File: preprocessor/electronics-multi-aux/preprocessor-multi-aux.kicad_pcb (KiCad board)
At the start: 2 copper layers, 17 x 24 mm, 19 parts, among them P1 ST-IN, P2 ST-OUT, P3 TH-IN, P4 TH-OUT, P5 AUX-IN, P6 LIGHT CONTROLLER, P7 AUX2-IN, P8 AUX3-IN, U1 MCP1703T-3302E/CB, U2 LPC811M001JDH16_TSSOP16

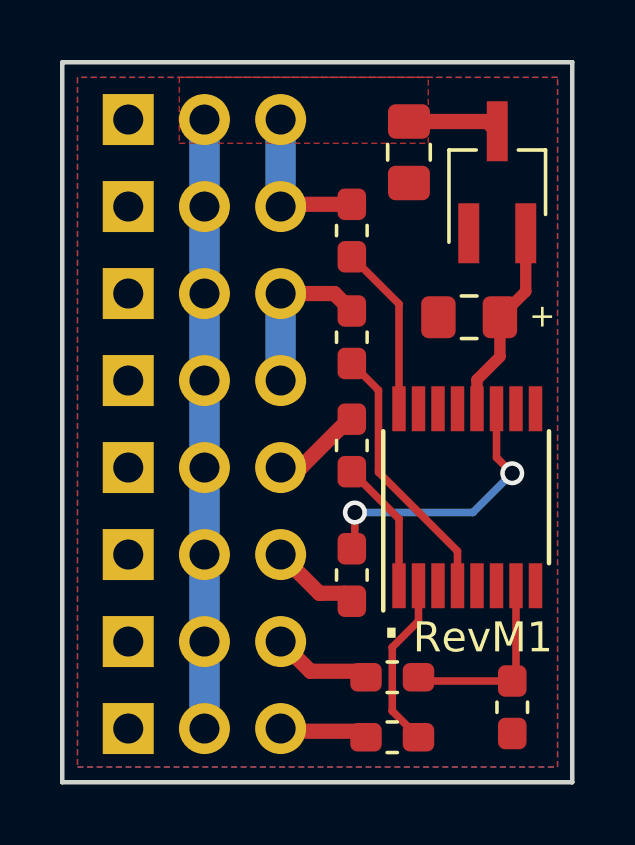
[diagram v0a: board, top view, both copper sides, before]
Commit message: Add to design doc and tweak PCB
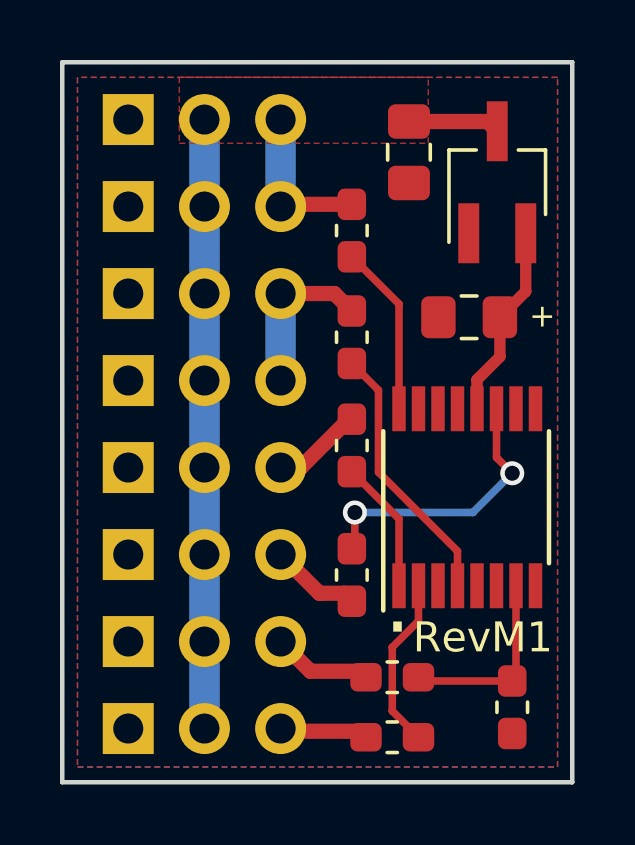
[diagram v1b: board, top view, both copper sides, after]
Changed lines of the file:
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@@
     (34 B.Paste user hide)
     (35 F.Paste user)
-    (36 B.SilkS user)
+    (36 B.SilkS user hide)
     (37 F.SilkS user)
     (38 B.Mask user hide)
@@
   )
   (setup
-    (last_trace_width 1.016)
+    (last_trace_width 0.254)
     (user_trace_width 0.381)
     (user_trace_width 0.508)
@@
     )
   )
-  (gr_text . (at 125.2728 60.2996) (layer F.SilkS)
+  (gr_text . (at 125.476 60.0964) (layer F.SilkS)
     (effects (font (size 2 2) (thickness 0.4)))
   )

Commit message: Update design doc
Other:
- board text added: "Note: pin headers spaced at 2.9mm to clear plug being wider on the top"
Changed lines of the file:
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@@
   (general
     (thickness 1.6)
-    (drawings 23)
+    (drawings 24)
     (tracks 56)
     (zones 0)
@@
     )
   )
+  (gr_text "Note: pin headers spaced at 2.9mm \nto clear plug being wider on the top" (at 98.552 53.2892) (layer Cmts.User)
+    (effects (font (size 1 1) (thickness 0.25)))
+  )
   (gr_text . (at 125.476 60.0964) (layer F.SilkS)

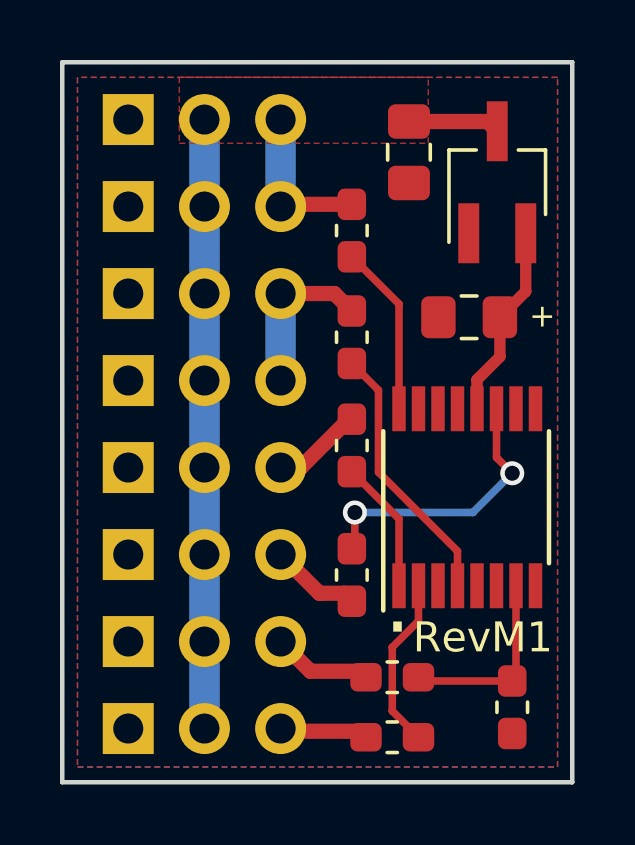
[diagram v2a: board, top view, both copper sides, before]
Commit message: Tweak tracks
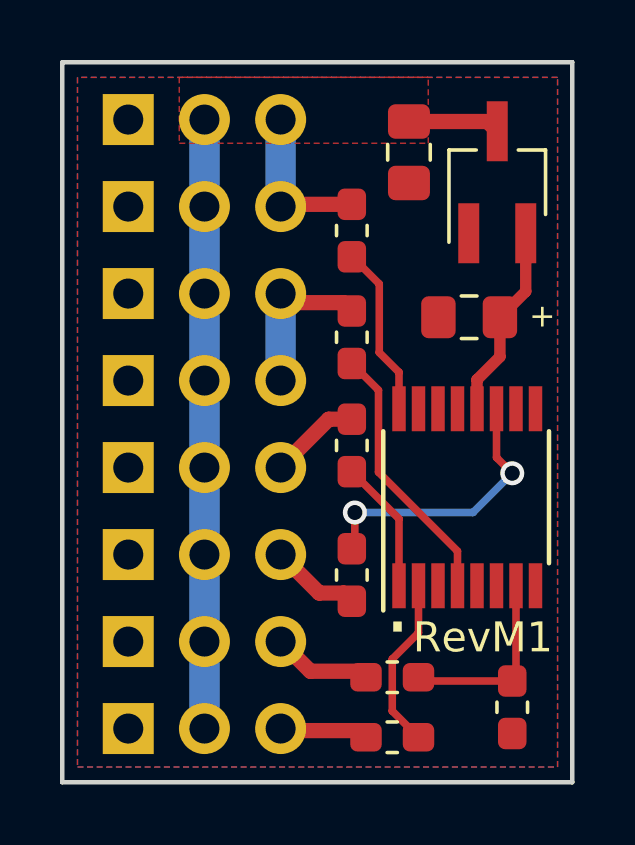
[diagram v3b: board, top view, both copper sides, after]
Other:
- rule pad_to_mask_clearance: 0.0508 -> 0.0254
- rule solder_mask_min_width: 0.0508 -> 0.0254
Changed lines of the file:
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@@
     (thickness 1.6)
     (drawings 24)
-    (tracks 56)
+    (tracks 60)
     (zones 0)
     (modules 19)
@@
     (34 B.Paste user hide)
     (35 F.Paste user)
-    (36 B.SilkS user hide)
+    (36 B.SilkS user)
     (37 F.SilkS user)
     (38 B.Mask user hide)
@@
     (pad_size 1.524 1.524)
     (pad_drill 0.762)
-    (pad_to_mask_clearance 0.0508)
-    (solder_mask_min_width 0.0508)
+    (pad_to_mask_clearance 0.0254)
+    (solder_mask_min_width 0.0254)
     (pad_to_paste_clearance_ratio -0.05)
     (aux_axis_origin 114.3 66.04)
@@
   (segment (start 128.125 52.6214) (end 128.8886 51.8578) (width 0.381) (layer F.Cu) (net 3))
   (segment (start 121.58 43.95) (end 121.58 46.85) (width 1.016) (layer B.Cu) (net 4))
+  (segment (start 123.952 46.7754) (end 121.6546 46.7754) (width 0.508) (layer F.Cu) (net 4))
   (segment (start 121.6546 46.7754) (end 121.58 46.85) (width 0.508) (layer F.Cu) (net 4))
-  (segment (start 123.952 46.7754) (end 121.6546 46.7754) (width 0.508) (layer F.Cu) (net 4))
   (segment (start 121.58 49.75) (end 121.58 52.65) (width 1.016) (layer B.Cu) (net 5))
-  (segment (start 123.3706 49.75) (end 123.952 50.3314) (width 0.508) (layer F.Cu) (net 5))
-  (segment (start 121.58 49.75) (end 123.3706 49.75) (width 0.508) (layer F.Cu) (net 5))
-  (segment (start 122.25 55.55) (end 121.58 55.55) (width 0.508) (layer F.Cu) (net 6))
-  (segment (start 123.952 53.9382) (end 123.8618 53.9382) (width 0.508) (layer F.Cu) (net 6))
-  (segment (start 123.8618 53.9382) (end 122.25 55.55) (width 0.508) (layer F.Cu) (net 6))
-  (segment (start 121.67 64.34) (end 121.58 64.25) (width 0.508) (layer F.Cu) (net 7))
-  (segment (start 124.425 64.54) (end 124.225 64.34) (width 0.508) (layer F.Cu) (net 7))
-  (segment (start 124.225 64.34) (end 121.67 64.34) (width 0.508) (layer F.Cu) (net 7))
-  (segment (start 125.525 50.0984) (end 125.525 53.59) (width 0.254) (layer F.Cu) (net 8))
-  (segment (start 123.952 48.5254) (end 125.525 50.0984) (width 0.254) (layer F.Cu) (net 8))
+  (segment (start 121.58 49.75) (end 121.88324 50.05324) (width 0.508) (layer F.Cu) (net 5))
+  (segment (start 123.67384 50.05324) (end 123.952 50.3314) (width 0.508) (layer F.Cu) (net 5))
+  (segment (start 121.88324 50.05324) (end 123.67384 50.05324) (width 0.508) (layer F.Cu) (net 5))
+  (segment (start 121.58 55.53928) (end 121.58 55.55) (width 0.508) (layer F.Cu) (net 6))
+  (segment (start 123.952 53.9382) (end 123.18108 53.9382) (width 0.508) (layer F.Cu) (net 6))
+  (segment (start 123.18108 53.9382) (end 121.58 55.53928) (width 0.508) (layer F.Cu) (net 6))
+  (segment (start 121.64788 64.31788) (end 121.58 64.25) (width 0.508) (layer F.Cu) (net 7))
+  (segment (start 124.425 64.54) (end 124.20288 64.31788) (width 0.508) (layer F.Cu) (net 7))
+  (segment (start 124.20288 64.31788) (end 121.64788 64.31788) (width 0.508) (layer F.Cu) (net 7))
+  (segment (start 125.525 52.373) (end 125.525 53.59) (width 0.254) (layer F.Cu) (net 8))
+  (segment (start 124.8664 49.4284) (end 124.8664 51.7144) (width 0.254) (layer F.Cu) (net 8))
+  (segment (start 124.8664 51.7144) (end 125.525 52.373) (width 0.254) (layer F.Cu) (net 8))
+  (segment (start 123.952 48.5254) (end 123.9634 48.5254) (width 0.254) (layer F.Cu) (net 8))
+  (segment (start 123.9634 48.5254) (end 124.8664 49.4284) (width 0.254) (layer F.Cu) (net 8))
   (segment (start 127.475 59.49) (end 127.475 58.3362) (width 0.254) (layer F.Cu) (net 9))
   (segment (start 127.475 58.3362) (end 124.841 55.7022) (width 0.254) (layer F.Cu) (net 9))
@@
   (segment (start 125.525 57.2612) (end 125.525 59.49) (width 0.254) (layer F.Cu) (net 10))
   (segment (start 123.952 55.6882) (end 125.525 57.2612) (width 0.254) (layer F.Cu) (net 10))
-  (segment (start 126.175 59.49) (end 126.175 60.665) (width 0.254) (layer F.Cu) (net 11))
-  (segment (start 126.175 60.665) (end 125.3 61.54) (width 0.254) (layer F.Cu) (net 11))
   (segment (start 125.3 63.665) (end 126.175 64.54) (width 0.254) (layer F.Cu) (net 11))
-  (segment (start 125.3 61.54) (end 125.3 63.665) (width 0.254) (layer F.Cu) (net 11))
-  (segment (start 122.8708 59.7408) (end 121.58 58.45) (width 0.508) (layer F.Cu) (net 12))
-  (segment (start 123.952 60.0062) (end 123.6866 59.7408) (width 0.508) (layer F.Cu) (net 12))
-  (segment (start 123.6866 59.7408) (end 122.8708 59.7408) (width 0.508) (layer F.Cu) (net 12))
+  (segment (start 125.3 61.93356) (end 125.3 63.665) (width 0.254) (layer F.Cu) (net 11))
+  (segment (start 126.175 59.49) (end 126.175 61.05856) (width 0.254) (layer F.Cu) (net 11))
+  (segment (start 126.175 61.05856) (end 125.3 61.93356) (width 0.254) (layer F.Cu) (net 11))
+  (segment (start 122.86318 59.73318) (end 121.58 58.45) (width 0.508) (layer F.Cu) (net 12))
+  (segment (start 123.952 60.0062) (end 123.67898 59.73318) (width 0.508) (layer F.Cu) (net 12))
+  (segment (start 123.67898 59.73318) (end 122.86318 59.73318) (width 0.508) (layer F.Cu) (net 12))
   (via (at 129.3 55.74) (size 0.8) (drill 0.5) (layers F.Cu B.Cu) (net 13))
   (segment (start 128.775 55.215) (end 128.775 53.59) (width 0.254) (layer F.Cu) (net 13))

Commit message: Add PCB thickness annotation
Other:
- board text added: "Thickness: 1mm"
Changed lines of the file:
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@@
   (general
     (thickness 1.6)
-    (drawings 24)
+    (drawings 25)
     (tracks 60)
     (zones 0)
@@
     )
   )
+  (gr_text "Thickness: 1mm" (at 99.06 39.37) (layer Cmts.User)
+    (effects (font (size 1.5 1.5) (thickness 0.3)))
+  )
   (gr_text "Note: pin headers spaced at 2.9mm \nto clear plug being wider on the top" (at 98.552 53.2892) (layer Cmts.User)
